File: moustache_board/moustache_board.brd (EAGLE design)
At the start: 50 x 40 mm, 129 parts, among them CON1 B7B-PH-K-S-SIDE, CON10 PINHEAD_1X01-2.54, CON11 PINHEAD_1X01-2.54, CON12 PINHEAD_1X02-2.54, CON13 PINHEAD_1X07-2, CON14 PINHEAD_1X07-2, CON2 B7B-PH-K-S-SIDE, CON3 PINHEAD_1X02-2.54, CON4 PINHEAD_1X01-2.54, CON5 PINHEAD_1X01-2.54, CON6 PINHEAD_1X01-2.54, CON7 PINHEAD_1X01-2.54, CON8 PINHEAD_1X01-2.54, CON9 PINHEAD_1X01-2.54, IC1 STM32F030K6TX-LQFP32(7X7), IC101 IRS44273L, IC201 IRS44273L, IC3 ST3485SOIC8, IC301 IRS44273L, IC6 MC74VHC1GT125, IC7 MC74VHC1GT125, IC8 LM317, Q101 N-FET-SOT23, Q201 N-FET-SOT23, Q301 N-FET-SOT23, Y1 16MHz

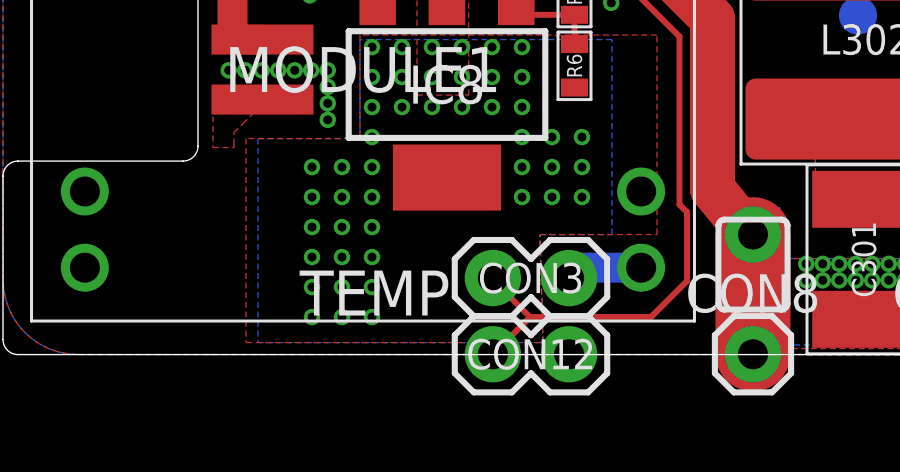
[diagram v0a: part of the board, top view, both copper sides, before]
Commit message: Minor changes
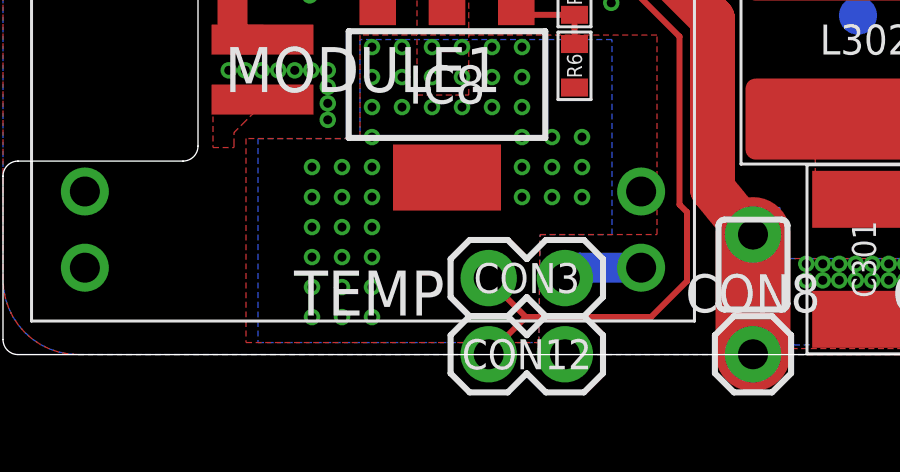
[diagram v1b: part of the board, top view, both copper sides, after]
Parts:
- moved CON12 0.14 mm to (-7.54, -20.0)
- moved CON3 0.14 mm to (-7.54, -17.4)
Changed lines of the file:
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@@
 <setting verticaltext="up"/>
 </settings>
-<grid distance="0.05" unitdist="mm" unit="mm" style="lines" multiple="2" display="yes" altdistance="0.5" altunitdist="mm" altunit="mm"/>
+<grid distance="0.01" unitdist="mm" unit="mm" style="lines" multiple="1" display="yes" altdistance="0.5" altunitdist="mm" altunit="mm"/>
 <layers>
 <layer number="1" name="Top" color="4" fill="1" visible="no" active="yes"/>
@@
 <text x="-10.325" y="8.075" size="1.5" layer="22" font="vector" ratio="15" rot="MR180" align="center">T</text>
 <text x="-12.95" y="-3.125" size="1.5" layer="22" font="vector" ratio="15" rot="MR0" align="center">I measure</text>
-<text x="-12.6" y="-17.95" size="1.5" layer="21" font="vector" ratio="15" align="center">TEMP</text>
+<text x="-12.79" y="-17.95" size="1.5" layer="21" font="vector" ratio="15" align="center">TEMP</text>
 <text x="9.45" y="-12.725" size="1.5" layer="22" font="vector" ratio="12" rot="MR0" align="center">d.e.palamarchuk@gmail.com</text>
 <wire x1="14.2" y1="14.95" x2="12.35" y2="14.95" width="0.2" layer="41"/>
@@
 <attribute name="TME#" value="RC0603FR-0710K" x="-6.2" y="1.3" size="1.778" layer="27" rot="R180" display="off"/>
 </element>
-<element name="CON3" library="pinhead" package="1X02-PTH-2.54" value="PINHEAD_1X02-2.54" x="-7.4" y="-17.45" rot="R180"/>
+<element name="CON3" library="pinhead" package="1X02-PTH-2.54" value="PINHEAD_1X02-2.54" x="-7.54" y="-17.45" rot="R180"/>
 <element name="C26" library="rc" package="C0603" value="100 nF" x="-6.2" y="0.05" rot="R180">
 <attribute name="PACKAGE" value="0603" x="-6.2" y="0.05" size="1.778" layer="27" rot="R180" display="off"/>
@@
 <element name="CON10" library="pinhead" package="1X01-PTH-2.54" value="PINHEAD_1X01-2.54" x="14.8" y="-19.99"/>
 <element name="CON11" library="pinhead" package="1X01-PTH-2.54" value="PINHEAD_1X01-2.54" x="7.4" y="-19.99"/>
-<element name="CON12" library="pinhead" package="1X02-PTH-2.54" value="PINHEAD_1X02-2.54" x="-7.4" y="-19.99" rot="R180"/>
+<element name="CON12" library="pinhead" package="1X02-PTH-2.54" value="PINHEAD_1X02-2.54" x="-7.54" y="-19.99" rot="R180"/>
 <element name="D5" library="pixel_masterlib" package="SMB" value="TVS_DIODE-SMB" x="-17.1" y="2.1">
 <attribute name="CHIPDIP#" value="8023193826" x="-17.1" y="2.1" size="1.778" layer="27" display="off"/>
@@
 <vertex x="-16.6" y="-11.9"/>
 </polygon>
-<wire x1="-6.13" y1="-17.45" x2="-5.784" y2="-17.104" width="1" layer="16"/>
+<wire x1="-6.27" y1="-17.45" x2="-5.784" y2="-17.104" width="1" layer="16"/>
 <wire x1="-5.784" y1="-17.104" x2="-3.729" y2="-17.104" width="1" layer="16"/>
 </signal>
@@
 <wire x1="-4.7" y1="3.175" x2="-4.7" y2="5.075" width="0.2" layer="1"/>
 <wire x1="-4.7" y1="5.075" x2="-3.6" y2="6.175" width="0.2" layer="1"/>
-<wire x1="-8.67" y1="-19.99" x2="-7.43" y2="-18.75" width="0.2" layer="1"/>
-<wire x1="-7.43" y1="-18.75" x2="-3.4" y2="-18.75" width="0.2" layer="1"/>
+<wire x1="-8.81" y1="-19.99" x2="-7.57" y2="-18.75" width="0.2" layer="1"/>
+<wire x1="-7.57" y1="-18.75" x2="-3.4" y2="-18.75" width="0.2" layer="1"/>
 <wire x1="-3.4" y1="-18.75" x2="-2.2" y2="-17.55" width="0.2" layer="1"/>
 <wire x1="-2.2" y1="-17.55" x2="-2.2" y2="-15.25" width="0.2" layer="1"/>
@@
 <wire x1="-6.925" y1="-0.875" x2="-6.925" y2="-2.475" width="0.2" layer="16"/>
 <wire x1="-6.925" y1="-2.475" x2="-5.8" y2="-3.6" width="0.2" layer="16"/>
-<wire x1="-7.43" y1="-18.75" x2="-8.67" y2="-17.51" width="0.2" layer="1"/>
-<wire x1="-8.67" y1="-17.51" x2="-8.67" y2="-17.45" width="0.2" layer="1"/>
+<wire x1="-7.57" y1="-18.75" x2="-8.81" y2="-17.51" width="0.2" layer="1"/>
+<wire x1="-8.81" y1="-17.51" x2="-8.81" y2="-17.45" width="0.2" layer="1"/>
 </signal>
 <signal name="LED1_PWM">
@@
 <polygon width="0.2" layer="1" thermals="no">
 <vertex x="-16.9" y="-19.6"/>
-<vertex x="-7" y="-19.6"/>
+<vertex x="-7.14" y="-19.6"/>
 <vertex x="-7.1" y="-16"/>
 <vertex x="-3.2" y="-16"/>
@@
 <polygon width="0.2" layer="16" thermals="no">
 <vertex x="-16.5" y="-19.6"/>
-<vertex x="-7" y="-19.6"/>
+<vertex x="-7.14" y="-19.6"/>
 <vertex x="-7.1" y="-16"/>
 <vertex x="-4.7" y="-16"/>
